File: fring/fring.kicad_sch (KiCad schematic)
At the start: 3 parts, among them J1 HLE-108-02-L-DV-K, J2 Conn_02x03_Odd_Even, J3 WE-RJ45_7499111447

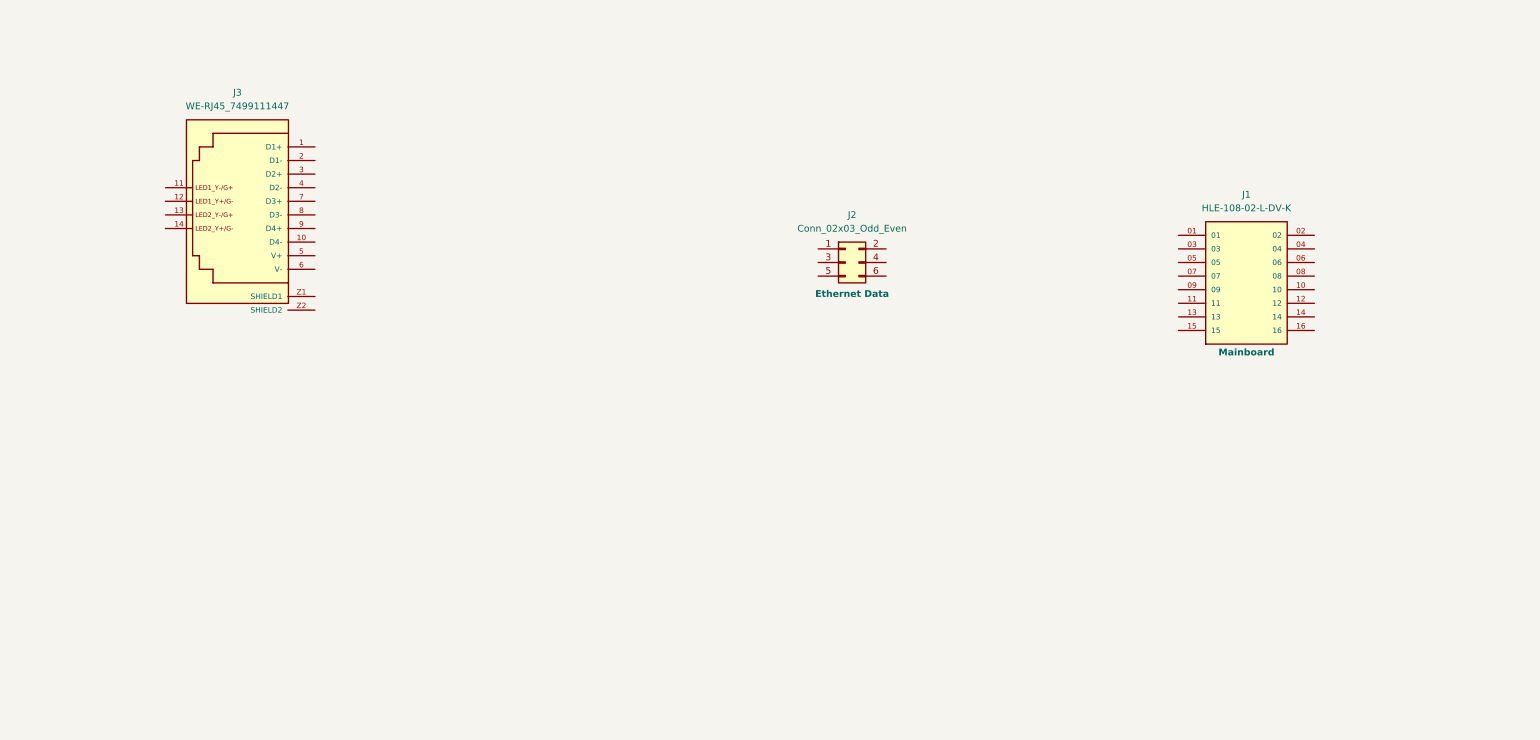
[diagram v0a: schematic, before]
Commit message: working on schematic layout
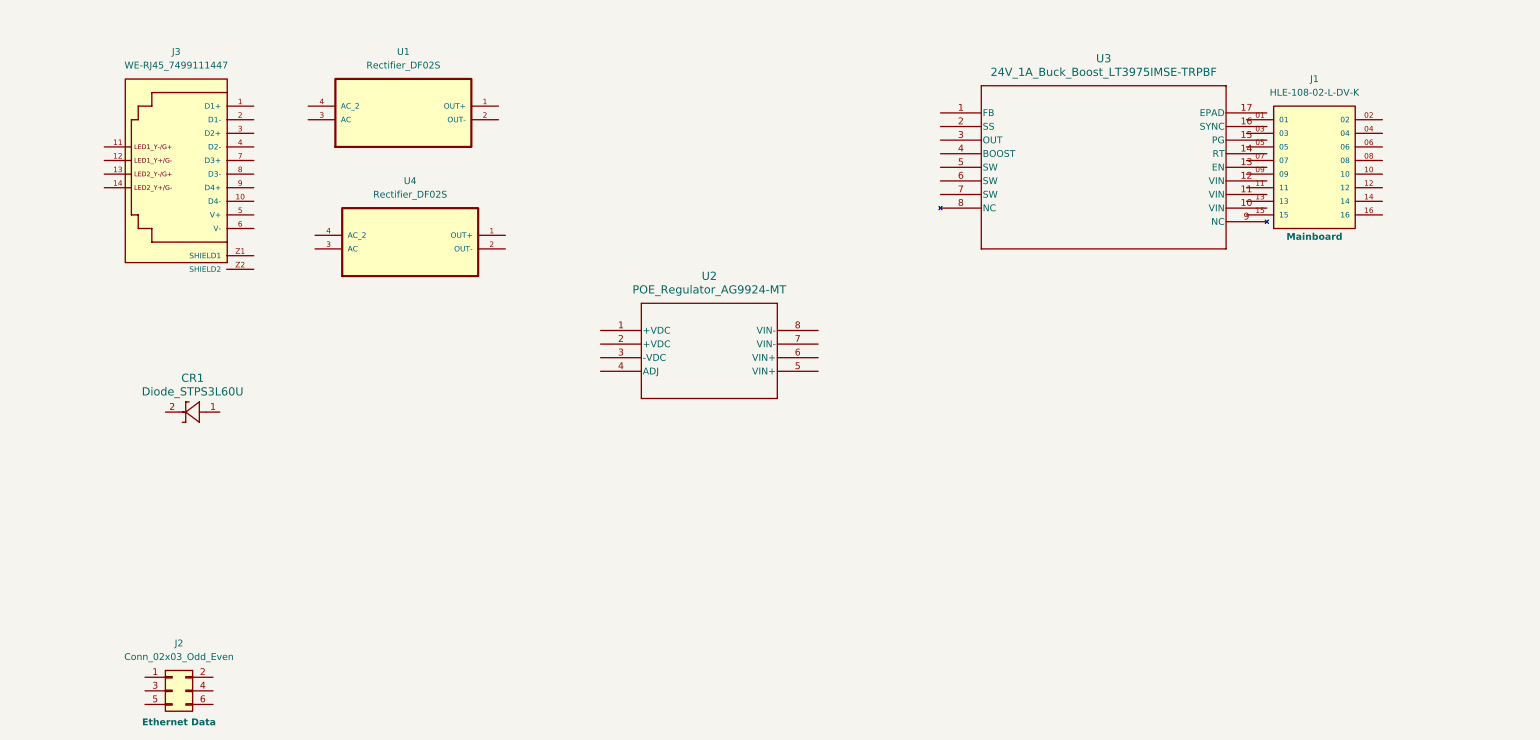
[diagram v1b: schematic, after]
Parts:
- added CR1: Diode_STPS3L60U, SMB_STM, symbol Fring Local:Diode_STPS3L60U
- added U1, U4: Rectifier_DF02S, DF02S:SOT508P985X260-4N, symbol Fring Local:Rectifier_DF02S
- added U2: POE_Regulator_AG9924-MT, AG9924-MT_SLV, symbol Fring Local:POE_Regulator_AG9924-MT
- added U3: 24V_1A_Buck_Boost_LT3975IMSE-TRPBF, MSOP-16_MSE_LIT, symbol Fring Local:24V_1A_Buck_Boost_LT3975IMSE-TRPBF
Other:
- moved on the sheet: J1, J2, J3

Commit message: started labeling schematics
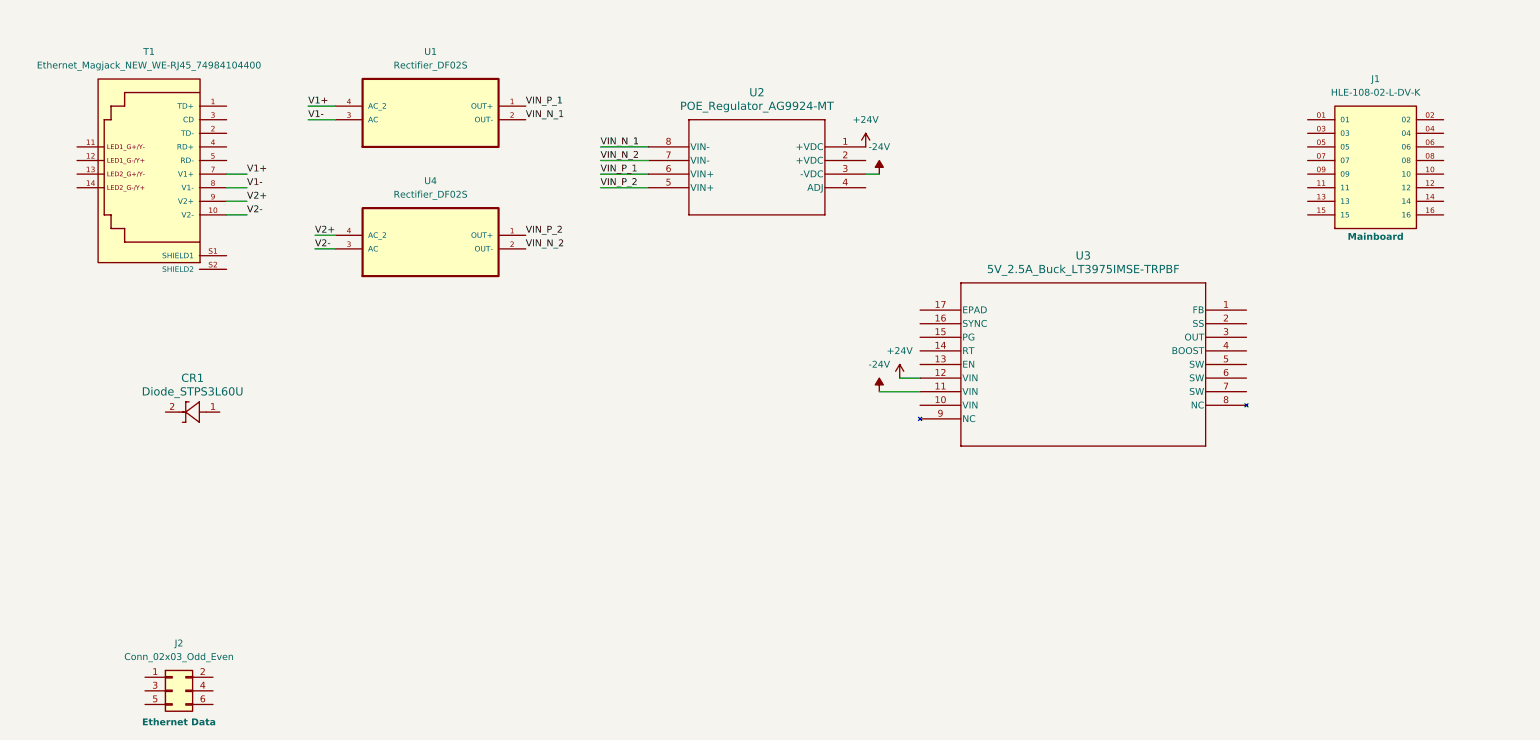
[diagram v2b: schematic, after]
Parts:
- removed J3: WE-RJ45_7499111447, MDFC Common:7499111447, symbol ModuleTemplate:WE-RJ45_7499111447
- added T1: Ethernet_Magjack_NEW_WE-RJ45_74984104400, WE-RJ45_74984104400:74984104400, symbol Fring Local:Ethernet_Magjack_NEW_WE-RJ45_74984104400
- U3: value 24V_1A_Buck_Boost_LT3975IMSE-TRPBF -> 5V_2.5A_Buck_LT3975IMSE-TRPBF
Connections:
- net VIN_P_1: now reaches U1.1 (OUT+)
- net VIN_P_1: now also U2.6 (VIN+)
- net VIN_N_1: now reaches U1.2 (OUT-)
- net VIN_N_1: now also U2.8 (VIN-)
- net V1-: now reaches U1.3 (AC)
- net V1-: now also T1.8 (V1-)
- net V1+: now reaches U1.4 (AC_2)
- net V1+: now also T1.7 (V1+)
- net +24V: now reaches U2.1 (+VDC)
- net +24V: now also U3.12 (VIN)
- net -24V: now reaches U2.3 (-VDC)
- net -24V: now also U3.11 (VIN)
- net VIN_P_2: now reaches U2.5 (VIN+)
- net VIN_P_2: now also U4.1 (OUT+)
- net VIN_N_2: now reaches U2.7 (VIN-)
- net VIN_N_2: now also U4.2 (OUT-)
- net V2-: now reaches U4.3 (AC)
- net V2-: now also T1.10 (V2-)
- net V2+: now reaches U4.4 (AC_2)
- net V2+: now also T1.9 (V2+)
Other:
- moved on the sheet: J1, U1, U2, U3, U4

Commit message: 90 percent done schematic
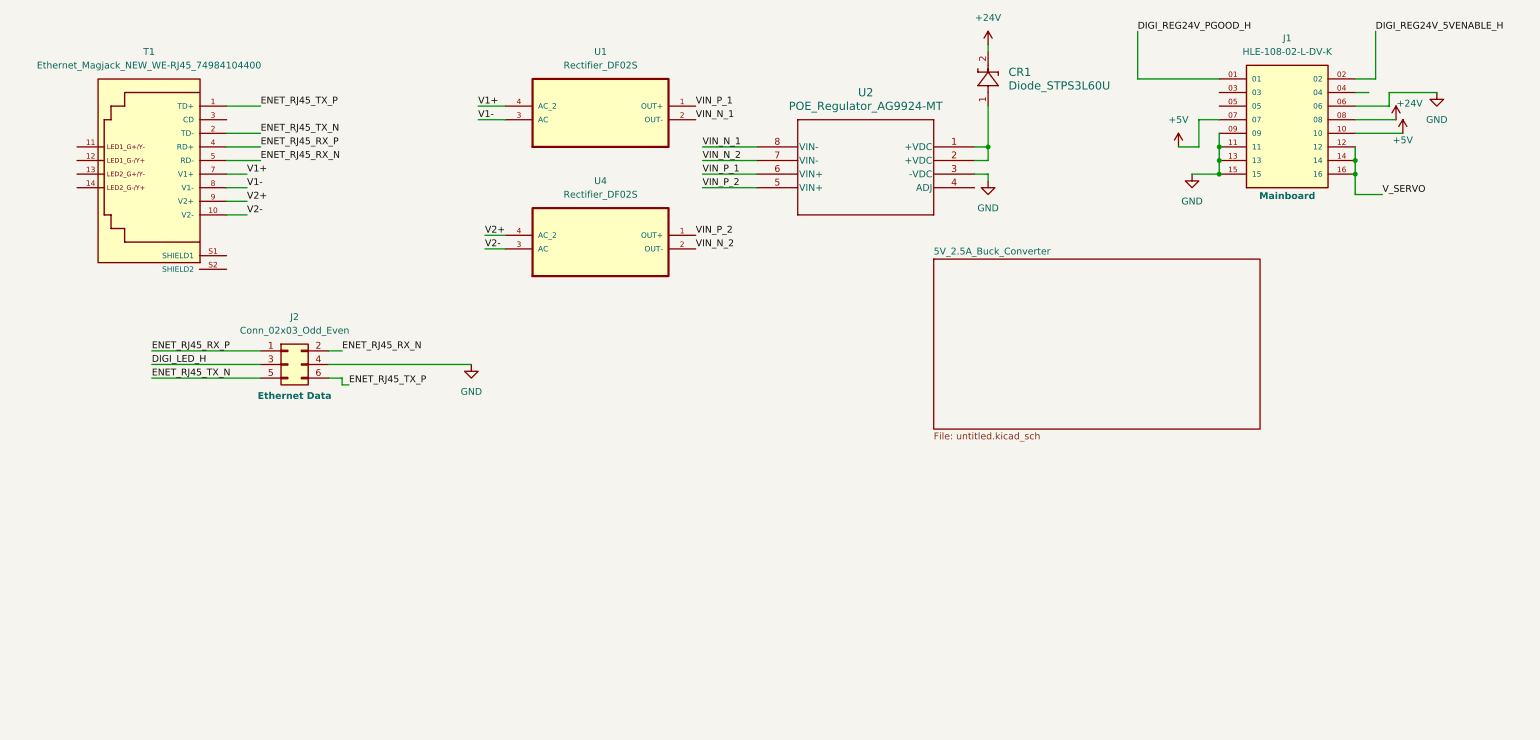
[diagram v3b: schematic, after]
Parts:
- removed U3: 5V_2.5A_Buck_LT3975IMSE-TRPBF, MSOP-16_MSE_LIT, symbol Fring Local:24V_1A_Buck_Boost_LT3975IMSE-TRPBF
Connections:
- net -24V is gone; now on net GND: U2.3 (-VDC)
- net +24V: now also CR1.2, J1.08; no longer U2.1 (+VDC)
- net at U2.2 (+VDC): now also CR1.1, U2.1 (+VDC)
- net ENET_RJ45_TX_P: now reaches T1.1 (TD+)
- net ENET_RJ45_TX_P: now also J2.6 (Pin_6)
- net ENET_RJ45_TX_N: now reaches T1.2 (TD-)
- net ENET_RJ45_TX_N: now also J2.5 (Pin_5)
- net ENET_RJ45_RX_P: now reaches T1.4 (RD+)
- net ENET_RJ45_RX_P: now also J2.1 (Pin_1)
- net ENET_RJ45_RX_N: now reaches T1.5 (RD-)
- net ENET_RJ45_RX_N: now also J2.2 (Pin_2)
- net DIGI_LED_H: now reaches J2.3 (Pin_3)
- net GND: now reaches J2.4 (Pin_4)
- net GND: now also J1.06, J1.09, J1.11, J1.13, J1.15
- net DIGI_REG24V_PGOOD_H: now reaches J1.01
- net DIGI_REG24V_5VENABLE_H: now reaches J1.02
- net +5V: now reaches J1.07
- net +5V: now also J1.10
- net V_SERVO: now reaches J1.12
- net V_SERVO: now also J1.14, J1.16
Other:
- added sheet 5V_2.5A_Buck_Converter (untitled.kicad_sch)
- moved on the sheet: CR1, J1, J2, U1, U2, U4
